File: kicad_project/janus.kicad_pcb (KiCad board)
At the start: 2 copper layers, 180.2 x 117.5 mm, 55 parts

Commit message: generated output
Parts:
- added D26: , ComboDiode, F.Cu at (159.7, 90.6)
- added D27: , ComboDiode, F.Cu at (161.1, 71.4)
- added D28: , ComboDiode, F.Cu at (131.2, 166.9)
- added D29: , ComboDiode, F.Cu at (150.2, 172.4)
- added D30: , ComboDiode, F.Cu at (170.1, 176.5)
- added D31: , ComboDiode, F.Cu at (187.0, 187.6)
- added S26: ks27, gateron-ks27, F.Cu at (150.3, 95.9)
- added S27: ks27, gateron-ks27, F.Cu at (151.7, 76.8)
- added S28: ks27, gateron-ks27, F.Cu at (126.8, 157.0)
- added S29: ks27, gateron-ks27, F.Cu at (147.3, 161.9)
- added S30: ks27, gateron-ks27, F.Cu at (168.7, 165.8)
- added S31: ks27, gateron-ks27, F.Cu at (187.1, 176.8)
- moved S5 164.4 mm to (50.0, 73.2), turned to 0 degrees
- moved D23 163.2 mm to (141.9, 70.1), turned to -94 degrees
- moved D5 162.5 mm to (59.0, 67.2), turned to -90 degrees
- moved D25 160.7 mm to (158.4, 109.7), turned to -94 degrees
- moved S25 158.5 mm to (149.0, 115.1), turned to -4 degrees
- moved S23 157.2 mm to (132.5, 75.4), turned to -4 degrees
- moved S9 147.8 mm to (69.2, 92.4), turned to 0 degrees
- moved D9 146.4 mm to (78.2, 86.4), turned to -90 degrees
- moved S10 145.5 mm to (69.2, 73.2), turned to 0 degrees
- moved D10 144.1 mm to (78.2, 67.2), turned to -90 degrees
- moved S13 134.0 mm to (89.9, 112.0), turned to -2 degrees
- moved D24 132.8 mm to (157.1, 128.9), turned to -94 degrees
- moved D13 132.4 mm to (99.1, 106.3), turned to -92 degrees
- moved S24 132.4 mm to (147.7, 134.2), turned to -4 degrees
- moved S14 130.9 mm to (90.6, 92.8), turned to -2 degrees
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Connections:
- net inner_cluster renamed index_number
- D1 pad 1: P9 -> (no net)
- D10 pad 1: P8 -> (no net)
- D10 pad 2: ring_bottom -> pinky_number
- D11 pad 1: P7 -> (no net)
- D11 pad 2: ring_home -> ring_mod
- D12 pad 1: P6 -> (no net)
- D12 pad 2: ring_top -> ring_bottom
- D13 pad 1: P9 -> (no net)
- D13 pad 2: middle_mod -> ring_home
- D14 pad 1: P8 -> (no net)
- D14 pad 2: middle_bottom -> ring_top
- D15 pad 1: P7 -> (no net)
- D15 pad 2: middle_home -> ring_number
- D16 pad 1: P6 -> (no net)
- D16 pad 2: middle_top -> middle_bottom
- D17 pad 1: P8 -> (no net)
- D17 pad 2: index_bottom -> middle_home
- D18 pad 1: P7 -> (no net)
- D18 pad 2: index_home -> middle_top
- D19 pad 1: P6 -> (no net)
- D19 pad 2: index_top -> middle_number
- D2 pad 1: P8 -> (no net)
- D20 pad 1: P8 -> (no net)
- D20 pad 2: inner_bottom -> index_bottom
- D21 pad 1: P7 -> (no net)
- D21 pad 2: inner_home -> index_home
- D22 pad 1: P6 -> (no net)
- D22 pad 2: inner_top -> index_top
- D23 pad 1: P9 -> (no net)
- D24 pad 1: P9 -> (no net)
- D24 pad 2: home_cluster -> inner_bottom
- D25 pad 1: P9 -> (no net)
- D25 pad 2: outer_cluster -> inner_home
- D3 pad 1: P7 -> (no net)
- D4 pad 1: P6 -> (no net)
- D5 pad 1: P9 -> (no net)
- D5 pad 2: pinky_mod -> outer_number
- D6 pad 1: P8 -> (no net)
- D6 pad 2: pinky_bottom -> pinky_mod
- D7 pad 1: P7 -> (no net)
- D7 pad 2: pinky_home -> pinky_bottom
- D8 pad 1: P6 -> (no net)
- D8 pad 2: pinky_top -> pinky_home
- D9 pad 1: P9 -> (no net)
- D9 pad 2: ring_mod -> pinky_top
- MCU1 pad : 14 -> P9
- OLED1 pad : O5 -> P1
- OLED1 pad 1: O1 -> (no net)
- OLED1 pad 2: O2 -> (no net)
- OLED1 pad 4: O4 -> (no net)
- OLED1 pad 5: O5 -> (no net)
- S1 pad 1: P20 -> (no net)
- S10 pad 1: P18 -> (no net)
- S10 pad 2: ring_bottom -> pinky_number
- S11 pad 1: P18 -> (no net)
- S11 pad 2: ring_home -> ring_mod
- S12 pad 1: P18 -> (no net)
- S12 pad 2: ring_top -> ring_bottom
- S13 pad 1: P15 -> (no net)
- S13 pad 2: middle_mod -> ring_home
- S14 pad 1: P15 -> (no net)
- S14 pad 2: middle_bottom -> ring_top
- S15 pad 1: P15 -> (no net)
- S15 pad 2: middle_home -> ring_number
- S16 pad 1: P15 -> (no net)
- S16 pad 2: middle_top -> middle_bottom
- S17 pad 1: P14 -> (no net)
- S17 pad 2: index_bottom -> middle_home
- S18 pad 1: P14 -> (no net)
- S18 pad 2: index_home -> middle_top
- S19 pad 1: P14 -> (no net)
- S19 pad 2: index_top -> middle_number
- S2 pad 1: P20 -> (no net)
- S20 pad 1: P16 -> (no net)
- S20 pad 2: inner_bottom -> index_bottom
- S21 pad 1: P16 -> (no net)
- S21 pad 2: inner_home -> index_home
- S22 pad 1: P16 -> (no net)
- S22 pad 2: inner_top -> index_top
- S23 pad 1: P14 -> (no net)
- S24 pad 1: P16 -> (no net)
- S24 pad 2: home_cluster -> inner_bottom
- S25 pad 1: P10 -> (no net)
- S25 pad 2: outer_cluster -> inner_home
- S3 pad 1: P20 -> (no net)
- S4 pad 1: P20 -> (no net)
- S5 pad 1: P19 -> (no net)
- S5 pad 2: pinky_mod -> outer_number
- S6 pad 1: P19 -> (no net)
- S6 pad 2: pinky_bottom -> pinky_mod
- S7 pad 1: P19 -> (no net)
- S7 pad 2: pinky_home -> pinky_bottom
- S8 pad 1: P19 -> (no net)
- S8 pad 2: pinky_top -> pinky_home
- S9 pad 1: P18 -> (no net)
- S9 pad 2: ring_mod -> pinky_top
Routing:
- net P20: track 294.8 -> 0.00 mm
- net P19: track 274.3 -> 0.00 mm
- net P9: track 261.4 -> 0.00 mm
- net P18: track 253.3 -> 0.00 mm
- net P15: track 233.2 -> 0.00 mm
- net P14: track 221.1 -> 0.00 mm
- net P16: track 200.2 -> 0.00 mm
- net P6: track 175.6 -> 0.00 mm
- net P8: track 169.0 -> 0.00 mm
- net P7: track 157.4 -> 0.00 mm
- net GND: track 118.4 -> 0.00 mm, vias 1 -> 0
- net P10: track 102.9 -> 0.00 mm, vias 1 -> 0
- net RST: track 77.7 -> 0.00 mm, vias 3 -> 0
- net RAW: track 72.8 -> 0.00 mm, vias 1 -> 0
- net P1: track 66.0 -> 0.00 mm, vias 2 -> 0
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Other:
- board size 180.2 x 117.5 mm -> 173.4 x 141.1 mm
- net class Default added: clearance 0.2, trace_width 0.25, via_dia 0.8, via_drill 0.4
- rule pad_to_mask_clearance: 0 -> 0.05

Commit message: generated output
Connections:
- D1 pad 1: (no net) -> P9
- D10 pad 1: (no net) -> P5
- D11 pad 1: (no net) -> P9
- D12 pad 1: (no net) -> P8
- D13 pad 1: (no net) -> P7
- D14 pad 1: (no net) -> P6
- D15 pad 1: (no net) -> P5
- D16 pad 1: (no net) -> P8
- D17 pad 1: (no net) -> P7
- D18 pad 1: (no net) -> P6
- D19 pad 1: (no net) -> P5
- D2 pad 1: (no net) -> P8
- D20 pad 1: (no net) -> P8
- D21 pad 1: (no net) -> P7
- D22 pad 1: (no net) -> P6
- D23 pad 1: (no net) -> P5
- D24 pad 1: (no net) -> P8
- D25 pad 1: (no net) -> P7
- D26 pad 1: (no net) -> P6
- D27 pad 1: (no net) -> P5
- D3 pad 1: (no net) -> P7
- D4 pad 1: (no net) -> P6
- D5 pad 1: (no net) -> P5
- D6 pad 1: (no net) -> P9
- D7 pad 1: (no net) -> P8
- D8 pad 1: (no net) -> P7
- D9 pad 1: (no net) -> P6
- S1 pad 1: (no net) -> P15
- S10 pad 1: (no net) -> P14
- S11 pad 1: (no net) -> P16
- S12 pad 1: (no net) -> P16
- S13 pad 1: (no net) -> P16
- S14 pad 1: (no net) -> P16
- S15 pad 1: (no net) -> P16
- S16 pad 1: (no net) -> P10
- S17 pad 1: (no net) -> P10
- S18 pad 1: (no net) -> P10
- S19 pad 1: (no net) -> P10
- S2 pad 1: (no net) -> P15
- S20 pad 1: (no net) -> P19
- S21 pad 1: (no net) -> P19
- S22 pad 1: (no net) -> P19
- S23 pad 1: (no net) -> P19
- S24 pad 1: (no net) -> P20
- S25 pad 1: (no net) -> P20
- S26 pad 1: (no net) -> P20
- S27 pad 1: (no net) -> P20
- S28 pad 1: (no net) -> P10
- S29 pad 1: P20 -> P19
- S3 pad 1: (no net) -> P15
- S30 pad 1: P19 -> P20
- S4 pad 1: (no net) -> P15
- S5 pad 1: (no net) -> P15
- S6 pad 1: (no net) -> P14
- S7 pad 1: (no net) -> P14
- S8 pad 1: (no net) -> P14
- S9 pad 1: (no net) -> P14

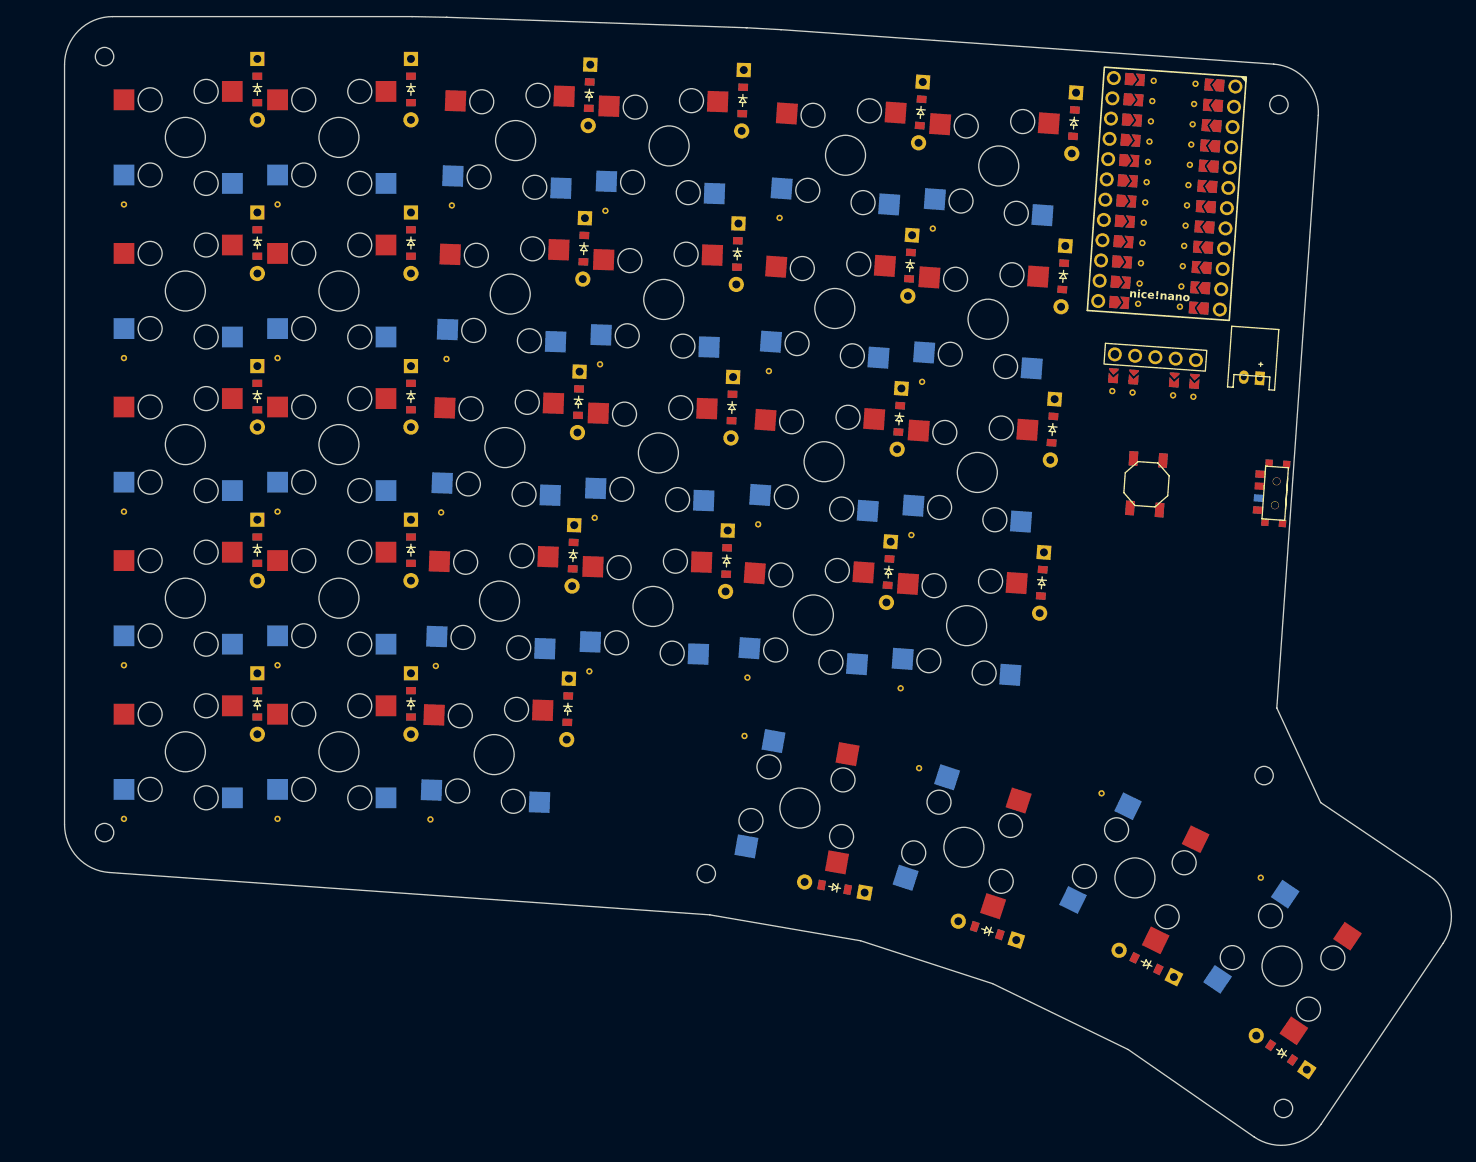
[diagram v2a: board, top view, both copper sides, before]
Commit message: final routing and generated gerbers
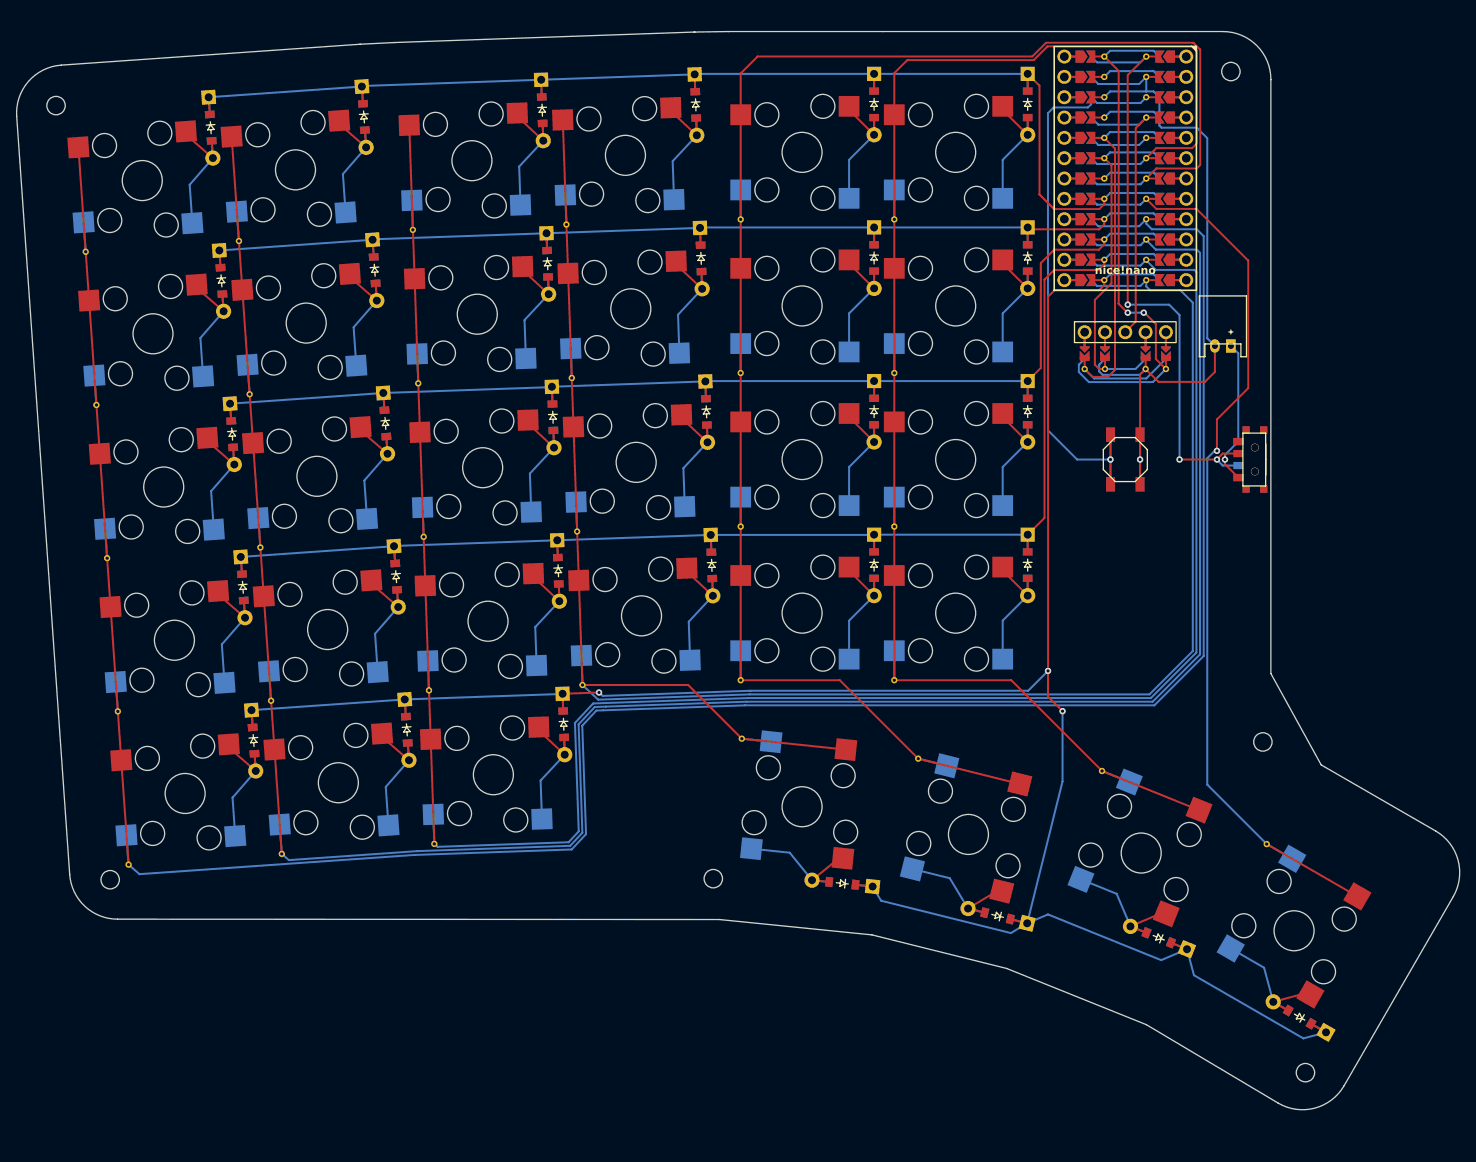
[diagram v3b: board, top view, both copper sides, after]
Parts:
- moved S5 7.62 mm to (44.6, 78.6), turned to 4 degrees
- moved D5 7.54 mm to (53.2, 72.0), turned to -86 degrees
- moved D10 6.81 mm to (72.3, 70.6), turned to -86 degrees
- moved S10 6.78 mm to (63.8, 77.3), turned to 4 degrees
- moved S4 6.71 mm to (46.0, 97.7), turned to 4 degrees
- moved D4 6.52 mm to (54.5, 91.1), turned to -86 degrees
- moved D27 6.24 mm to (155.3, 69.1), turned to -90 degrees
- moved D15 6.17 mm to (94.6, 69.8), turned to -88 degrees
- moved MCU1 6.09 mm to (167.5, 77.1), turned to 0 degrees
- moved S15 6.01 mm to (85.8, 76.1), turned to 2 degrees
- moved S3 5.95 mm to (47.3, 116.9), turned to 4 degrees
- moved D23 5.91 mm to (136.1, 69.1), turned to -90 degrees
- moved D19 5.90 mm to (113.8, 69.1), turned to -88 degrees
- moved OLED1 5.85 mm to (167.5, 81.1), turned to 0 degrees
- moved S9 5.73 mm to (65.1, 96.4), turned to 4 degrees
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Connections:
- MCU1 pad : P9 -> 17
- OLED1 pad : P1 -> P2
- OLED1 pad 1: (no net) -> O1
- OLED1 pad 2: (no net) -> O2
- OLED1 pad 4: (no net) -> O4
- OLED1 pad 5: (no net) -> O5
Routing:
- net P15: track 0.00 -> 331.6 mm
- net P14: track 0.00 -> 308.3 mm
- net P9: track 0.00 -> 292.9 mm, vias 0 -> 3
- net P16: track 0.00 -> 285.4 mm
- net P10: track 0.00 -> 264.3 mm
- net P19: track 0.00 -> 224.0 mm
- net P20: track 0.00 -> 205.2 mm
- net P8: track 0.00 -> 175.1 mm
- net P5: track 0.00 -> 163.0 mm
- net P7: track 0.00 -> 159.8 mm
- net P6: track 0.00 -> 146.8 mm
- net P18: track 0.00 -> 120.2 mm, vias 0 -> 1
- net GND: track 0.00 -> 109.3 mm, vias 0 -> 1
- net RST: track 0.00 -> 77.3 mm, vias 0 -> 1
- net RAW: track 0.00 -> 76.8 mm, vias 0 -> 3
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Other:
- board size 173.4 x 141.1 mm -> 180.4 x 134.8 mm
- net class Default removed
- rule pad_to_mask_clearance: 0.05 -> 0
